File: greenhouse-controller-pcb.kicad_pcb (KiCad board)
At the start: 2 copper layers, 1 part, among them J4 JTAG Interface

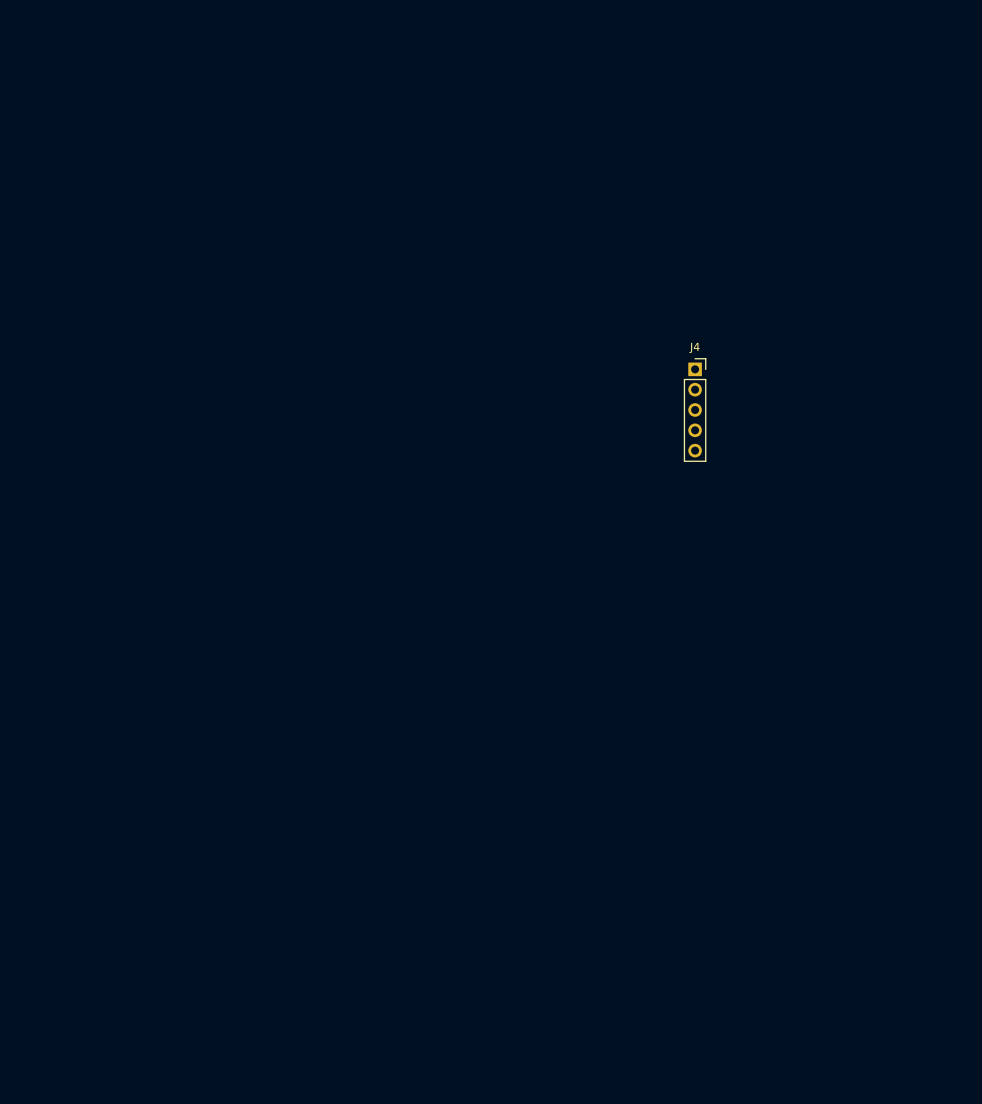
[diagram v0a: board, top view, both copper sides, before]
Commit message: version 1
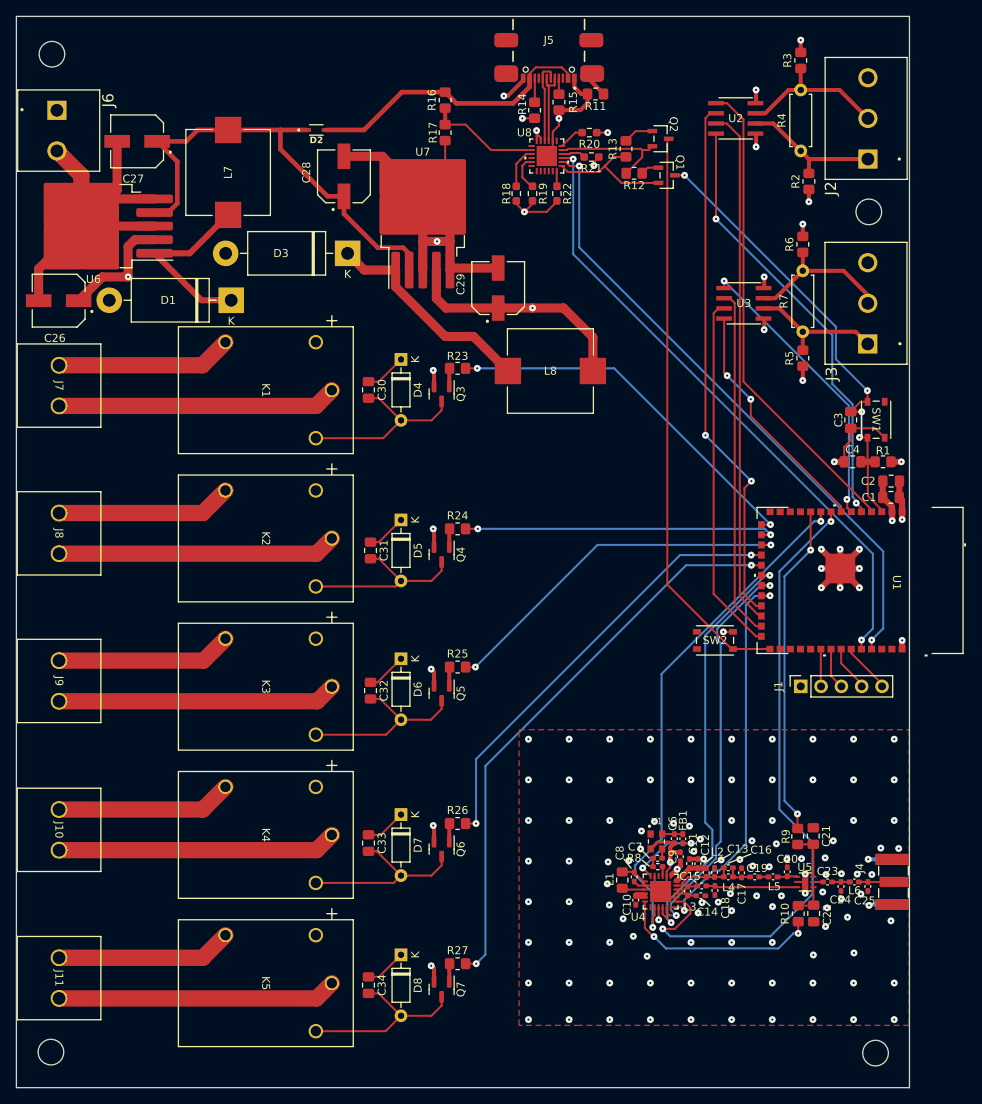
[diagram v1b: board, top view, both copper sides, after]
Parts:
- added C1: 22uF, Capacitor_SMD:C_0805_2012Metric_Pad1.18x1.45mm_HandSolder, F.Cu at (189.6, 87.1)
- added C10: 100nF, Capacitor_SMD:C_0402_1005Metric_Pad0.74x0.62mm_HandSolder, F.Cu at (157.7, 137.5)
- added C11: 47nF, Capacitor_SMD:C_0402_1005Metric_Pad0.74x0.62mm_HandSolder, F.Cu at (164.4, 132.9)
- added C12: 47pF, Capacitor_SMD:C_0402_1005Metric_Pad0.74x0.62mm_HandSolder, F.Cu at (165.4, 132.9)
- added C13: 8.2pF, Capacitor_SMD:C_0402_1005Metric_Pad0.74x0.62mm_HandSolder, F.Cu at (167.5, 134.0)
- added C14: 1.8pF, Capacitor_SMD:C_0402_1005Metric_Pad0.74x0.62mm_HandSolder, F.Cu at (165.8, 136.9)
- added C15: 2.4pF, Capacitor_SMD:C_0402_1005Metric_Pad0.74x0.62mm_HandSolder, F.Cu at (165.9, 135.7)
- added C16: 3.3pF, Capacitor_SMD:C_0402_1005Metric_Pad0.74x0.62mm_HandSolder, F.Cu at (169.3, 133.4)
- added C17: 8.2pF, Capacitor_SMD:C_0402_1005Metric_Pad0.74x0.62mm_HandSolder, F.Cu at (170.9, 134.1)
- added C18: 1.8pF, Capacitor_SMD:C_0402_1005Metric_Pad0.74x0.62mm_HandSolder, F.Cu at (167.6, 136.3)
- added C19: 39pF, Capacitor_SMD:C_0402_1005Metric_Pad0.74x0.62mm_HandSolder, F.Cu at (172.6, 134.6)
- added C2: 0.1uF, Capacitor_SMD:C_0805_2012Metric_Pad1.18x1.45mm_HandSolder, F.Cu at (189.6, 85.1)
- added C20: 3.0pF, Capacitor_SMD:C_0402_1005Metric_Pad0.74x0.62mm_HandSolder, F.Cu at (176.6, 133.9)
- added C21: 100nF, Capacitor_SMD:C_0805_2012Metric_Pad1.18x1.45mm_HandSolder, F.Cu at (179.9, 129.5)
- added C22: 100nF, Capacitor_SMD:C_0805_2012Metric_Pad1.18x1.45mm_HandSolder, F.Cu at (179.9, 139.1)
- added C23: 39pF, Capacitor_SMD:C_0402_1005Metric_Pad0.74x0.62mm_HandSolder, F.Cu at (181.7, 135.2)
- added C24: 3.3pF, Capacitor_SMD:C_0402_1005Metric_Pad0.74x0.62mm_HandSolder, F.Cu at (183.3, 135.8)
- added C25: 3.3pF, Capacitor_SMD:C_0402_1005Metric_Pad0.74x0.62mm_HandSolder, F.Cu at (186.7, 135.8)
- added C26: 120 uF, Library:CAP_EEEFNV121XUP, F.Cu at (85.5, 62.5)
- added C27: 120 uF, Library:CAP_EEEFNV121XUP, F.Cu at (95.4, 42.6)
- added C28: 120 uF, Library:CAP_EEEFNV121XUP, F.Cu at (121.2, 47.0)
- added C29: 120 uF, Library:CAP_EEEFNV121XUP, F.Cu at (140.5, 61.0)
- added C3: 1uF, Capacitor_SMD:C_0805_2012Metric_Pad1.18x1.45mm_HandSolder, F.Cu at (184.6, 77.4)
- added C30: 0.1 uF, Capacitor_SMD:C_0805_2012Metric_Pad1.18x1.45mm_HandSolder, F.Cu at (124.3, 73.7)
- added C31: 0.1 uF, Capacitor_SMD:C_0805_2012Metric_Pad1.18x1.45mm_HandSolder, F.Cu at (124.5, 93.8)
- added C32: 0.1 uF, Capacitor_SMD:C_0805_2012Metric_Pad1.18x1.45mm_HandSolder, F.Cu at (124.5, 111.3)
- added C33: 0.1 uF, Capacitor_SMD:C_0805_2012Metric_Pad1.18x1.45mm_HandSolder, F.Cu at (124.3, 130.3)
- added C34: 0.1 uF, Capacitor_SMD:C_0805_2012Metric_Pad1.18x1.45mm_HandSolder, F.Cu at (124.3, 148.1)
- added C4: 0.1uF, Capacitor_SMD:C_0805_2012Metric_Pad1.18x1.45mm_HandSolder, F.Cu at (184.8, 82.7)
- added C6: 100nF, Capacitor_SMD:C_0402_1005Metric_Pad0.74x0.62mm_HandSolder, F.Cu at (162.5, 129.8)
- added C7: 10pF, Capacitor_SMD:C_0402_1005Metric_Pad0.74x0.62mm_HandSolder, F.Cu at (160.4, 132.2)
- added C8: 470nF, Capacitor_SMD:C_0402_1005Metric_Pad0.74x0.62mm_HandSolder, F.Cu at (157.5, 134.6)
- added C9: 10nF, Capacitor_SMD:C_0402_1005Metric_Pad0.74x0.62mm_HandSolder, F.Cu at (163.3, 132.0)
- added D1: 1N5822, Diode_THT:D_DO-201AD_P15.24mm_Horizontal, F.Cu at (107.1, 62.5)
- added D2: BAT760-7, Library:SOD2513X120N, F.Cu at (117.8, 41.2)
- added D3: 1N5822, Diode_THT:D_DO-201AD_P15.24mm_Horizontal, F.Cu at (121.7, 56.6)
- added D4: 1N4148, Diode_THT:D_DO-35_SOD27_P7.62mm_Horizontal, F.Cu at (128.3, 69.9)
- added D5: 1N4148, Diode_THT:D_DO-35_SOD27_P7.62mm_Horizontal, F.Cu at (128.3, 89.9)
- added D6: 1N4148, Diode_THT:D_DO-35_SOD27_P7.62mm_Horizontal, F.Cu at (128.3, 107.3)
- added D7: 1N4148, Diode_THT:D_DO-35_SOD27_P7.62mm_Horizontal, F.Cu at (128.3, 126.8)
- added D8: 1N4148, Diode_THT:D_DO-35_SOD27_P7.62mm_Horizontal, F.Cu at (128.3, 144.3)
- added FB1: 10Ω@100MHz, Inductor_SMD:L_0402_1005Metric_Pad0.77x0.64mm_HandSolder, F.Cu at (163.6, 129.8)
- added J1: JTAG Interface, Connector_PinSocket_2.54mm:PinSocket_1x05_P2.54mm_Vertical, F.Cu at (178.3, 110.7)
- added J10: Relay 5 Ctrl., Library:TB004-508-02BE_CUD, F.Cu at (85.6, 126.1)
- added J11: Relay 3 Ctrl., Library:TB004-508-02BE_CUD, F.Cu at (85.6, 144.7)
- added J2: Screw_Terminal_01x03, Library:CUI_TB007-508-03BE, F.Cu at (186.7, 44.8)
- added J3: Screw_Terminal_01x03, Library:CUI_TB007-508-03BE, F.Cu at (186.7, 67.9)
- added J5: USB4105GFA, Library:GCT_USB4105GFA, F.Cu at (146.8, 30.0)
- added J6: POWER IN, Library:CUI_TB007-508-02BE, F.Cu at (85.3, 38.7)
- added J7: Relay 1 Ctrl., Library:TB004-508-02BE_CUD, F.Cu at (85.6, 70.6)
- added J8: Relay 4 Ctrl., Library:TB004-508-02BE_CUD, F.Cu at (85.6, 89.1)
- added J9: Relay 2 Ctrl., Library:TB004-508-02BE_CUD, F.Cu at (85.6, 107.5)
- added K1: G5LE-1A4 DC12, Library:RELAY_G5LE-1A DC5_OMR, F.Cu at (103.2, 73.7)
- added K2: G5LE-1A4 DC12, Library:RELAY_G5LE-1A DC5_OMR, F.Cu at (103.2, 92.3)
- added K3: G5LE-1A4 DC12, Library:RELAY_G5LE-1A DC5_OMR, F.Cu at (103.2, 110.8)
- added K4: G5LE-1A4 DC12, Library:RELAY_G5LE-1A DC5_OMR, F.Cu at (103.2, 129.3)
- added K5: G5LE-1A4 DC12, Library:RELAY_G5LE-1A DC5_OMR, F.Cu at (103.2, 147.8)
- added L1: 15uH, Inductor_SMD:L_0805_2012Metric_Pad1.15x1.40mm_HandSolder, F.Cu at (156.0, 135.0)
- added L2: 47nH, Inductor_SMD:L_0402_1005Metric_Pad0.77x0.64mm_HandSolder, F.Cu at (166.5, 134.0)
- added L3: 15nH, Inductor_SMD:L_0402_1005Metric_Pad0.77x0.64mm_HandSolder, F.Cu at (164.2, 136.3)
- added L4: 2.2nH, Inductor_SMD:L_0402_1005Metric_Pad0.77x0.64mm_HandSolder, F.Cu at (169.3, 134.6)
- added L5: 9.1nH, Inductor_SMD:L_0402_1005Metric_Pad0.77x0.64mm_HandSolder, F.Cu at (174.8, 134.6)
- added L6: 9.1nH, Inductor_SMD:L_0402_1005Metric_Pad0.77x0.64mm_HandSolder, F.Cu at (185.0, 135.2)
- added L7: 68 uH, Library:DR1050, F.Cu at (106.7, 46.5)
- added L8: 68 uH, Library:DR1050, F.Cu at (147.0, 71.3)
- added Q1: SS8050-G, Library:TRAN_SS8050-G_CIP, F.Cu at (161.5, 46.9)
- added Q2: SS8050-G, Library:TRAN_SS8050-G_CIP, F.Cu at (160.8, 42.3)
- added Q3: 2N7002, Package_TO_SOT_SMD:SOT-23, F.Cu at (133.4, 74.2)
- added Q4: 2N7002, Package_TO_SOT_SMD:SOT-23, F.Cu at (133.4, 94.3)
- added Q5: 2N7002, Package_TO_SOT_SMD:SOT-23, F.Cu at (133.4, 111.6)
- added Q6: 2N7002, Package_TO_SOT_SMD:SOT-23, F.Cu at (133.4, 131.1)
- added Q7: 2N7002, Package_TO_SOT_SMD:SOT-23, F.Cu at (133.4, 148.6)
- added R1: 10kΩ, Resistor_SMD:R_0805_2012Metric_Pad1.20x1.40mm_HandSolder, F.Cu at (188.6, 82.7)
- added R10: 100Ω, Resistor_SMD:R_0805_2012Metric_Pad1.20x1.40mm_HandSolder, F.Cu at (178.0, 139.2)
- added R11: 1MΩ, Resistor_SMD:R_0805_2012Metric_Pad1.20x1.40mm_HandSolder, F.Cu at (152.7, 36.7)
- added R12: 10k, Resistor_SMD:R_0805_2012Metric_Pad1.20x1.40mm_HandSolder, F.Cu at (157.5, 46.6)
- added R13: 10k, Resistor_SMD:R_0805_2012Metric_Pad1.20x1.40mm_HandSolder, F.Cu at (156.5, 43.6)
- added R14: 5.11kΩ, Resistor_SMD:R_0805_2012Metric_Pad1.20x1.40mm_HandSolder, F.Cu at (145.0, 38.7)
- added R15: 5.11kΩ, Resistor_SMD:R_0805_2012Metric_Pad1.20x1.40mm_HandSolder, F.Cu at (148.1, 37.7)
- added R16: 22.1kΩ, Resistor_SMD:R_0805_2012Metric_Pad1.20x1.40mm_HandSolder, F.Cu at (133.9, 37.5)
- added R17: 47.5kΩ, Resistor_SMD:R_0805_2012Metric_Pad1.20x1.40mm_HandSolder, F.Cu at (133.9, 41.5)
- added R18: 2kΩ, Resistor_SMD:R_0603_1608Metric_Pad0.98x0.95mm_HandSolder, F.Cu at (142.7, 49.1)
- added R19: 2kΩ, Resistor_SMD:R_0603_1608Metric_Pad0.98x0.95mm_HandSolder, F.Cu at (144.8, 49.1)
- added R2: 1k, Resistor_SMD:R_0805_2012Metric_Pad1.20x1.40mm_HandSolder, F.Cu at (179.3, 47.6)
- added R20: 2kΩ, Resistor_SMD:R_0603_1608Metric_Pad0.98x0.95mm_HandSolder, F.Cu at (151.9, 41.5)
- added R21: 2kΩ, Resistor_SMD:R_0603_1608Metric_Pad0.98x0.95mm_HandSolder, F.Cu at (152.1, 44.6)
- added R22: 2kΩ, Resistor_SMD:R_0603_1608Metric_Pad0.98x0.95mm_HandSolder, F.Cu at (147.8, 49.1)
- added R23: 100Ω, Resistor_SMD:R_0805_2012Metric_Pad1.20x1.40mm_HandSolder, F.Cu at (135.4, 71.0)
- added R24: 100Ω, Resistor_SMD:R_0805_2012Metric_Pad1.20x1.40mm_HandSolder, F.Cu at (135.4, 91.1)
- added R25: 100Ω, Resistor_SMD:R_0805_2012Metric_Pad1.20x1.40mm_HandSolder, F.Cu at (135.4, 108.3)
- added R26: 100Ω, Resistor_SMD:R_0805_2012Metric_Pad1.20x1.40mm_HandSolder, F.Cu at (135.4, 127.9)
- added R27: 100Ω, Resistor_SMD:R_0805_2012Metric_Pad1.20x1.40mm_HandSolder, F.Cu at (135.4, 145.4)
- added R3: 1k, Resistor_SMD:R_0805_2012Metric_Pad1.20x1.40mm_HandSolder, F.Cu at (178.3, 32.5)
- added R4: 120, Resistor_THT:R_Axial_DIN0207_L6.3mm_D2.5mm_P7.62mm_Horizontal, F.Cu at (178.3, 43.8)
- added R5: 1k, Resistor_SMD:R_0805_2012Metric_Pad1.20x1.40mm_HandSolder, F.Cu at (178.6, 69.7)
- added R6: 1k, Resistor_SMD:R_0805_2012Metric_Pad1.20x1.40mm_HandSolder, F.Cu at (178.6, 55.5)
- added R7: 120, Resistor_THT:R_Axial_DIN0207_L6.3mm_D2.5mm_P7.62mm_Horizontal, F.Cu at (178.6, 66.4)
- added R8: 220Ω, Resistor_SMD:R_0402_1005Metric_Pad0.72x0.64mm_HandSolder, F.Cu at (160.4, 133.3)
- added R9: 100Ω, Resistor_SMD:R_0805_2012Metric_Pad1.20x1.40mm_HandSolder, F.Cu at (177.9, 129.5)
- added REF**: MountingHole_3.2mm_M3, MountingHole:MountingHole_3.2mm_M3, F.Cu at (187.7, 156.6)
- added REF**: MountingHole_3.2mm_M3, MountingHole:MountingHole_3.2mm_M3, F.Cu at (186.8, 51.4)
- added REF**: MountingHole_3.2mm_M3, MountingHole:MountingHole_3.2mm_M3, F.Cu at (84.6, 156.5)
- added REF**: MountingHole_3.2mm_M3, MountingHole:MountingHole_3.2mm_M3, F.Cu at (84.7, 31.7)
- added SW1: RESET, Library:SW4_PTS815 SJM 250 SMTR LFS_CNK, F.Cu at (187.7, 77.4)
- added SW2: Boot mode, Library:SW4_PTS815 SJM 250 SMTR LFS_CNK, F.Cu at (167.6, 105.0)
- added U1: ~, Library:ESP32-S3-WROOM-1_EXP, F.Cu at (185.7, 97.5)
- added U2: ADM3483ARZ, Library:R_8_ADI, F.Cu at (170.2, 39.8)
- added U3: ADM3483ARZ, Library:R_8_ADI, F.Cu at (171.2, 62.9)
- added U4: SX1262IMLTRT, Library:QFN24_4X4_SEM, F.Cu at (160.8, 136.4)
- added U5: CG2179M2, Library:MINISO6_CG21_CEL, F.Cu at (178.9, 135.2)
- added U6: LM2595S-5, Package_TO_SOT_SMD:TO-263-5_TabPin3, F.Cu at (89.9, 53.2)
- added U7: LM2595S-3.3, Package_TO_SOT_SMD:TO-263-5_TabPin3, F.Cu at (131.1, 51.1)
- added U8: CP2102N-A02-GQFN24R, Library:QFN24_SIL, F.Cu at (146.6, 44.5)
- added Y1: 32 MHz, Library:OSC_ECS-TXO-2520-33-320-AN-TR, F.Cu at (160.3, 130.1)
- J4: value JTAG Interface -> SMA; footprint Connector_PinSocket_2.54mm:PinSocket_1x05_P2.54mm_Vertical -> Connector_Coaxial:SMA_Samtec_SMA-J-P-X-ST-EM1_EdgeMount
- moved J4 68.6 mm to (189.8, 135.2), turned to 90 degrees
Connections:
- J4 pad 1: GNDREF -> Net-(J4-In)
- J4 pad 2: /JTAG_TCK -> GNDREF
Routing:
- net GNDREF: track 0.00 -> 211.1 mm, vias 0 -> 135
- net LoRa_SPI_CS: track 0.00 -> 80.6 mm, vias 0 -> 2
- net ESP32_UART_TX: track 0.00 -> 79.1 mm, vias 0 -> 2
- net ESP32_UART_RX: track 0.00 -> 78.8 mm, vias 0 -> 2
- net BOOT_MODE: track 0.00 -> 72.0 mm
- net RELAY_5: track 0.00 -> 71.4 mm, vias 0 -> 2
- net RS-485_1_RX_EN: track 0.00 -> 66.5 mm, vias 0 -> 2
- net LoRa_BUSY: track 0.00 -> 65.6 mm, vias 0 -> 2
- net RS-485_1_TX_EN: track 0.00 -> 64.9 mm
- net RS-485_1_RX: track 0.00 -> 59.9 mm
- net +3.3V: track 0.00 -> 59.3 mm, vias 0 -> 13
- net EN: track 0.00 -> 59.1 mm, vias 0 -> 4
- net +5V: track 0.00 -> 58.7 mm
- net RELAY_4: track 0.00 -> 55.6 mm, vias 0 -> 2
- net RS-485_1_TX: track 0.00 -> 54.8 mm, vias 0 -> 2
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- added copper zone on In2.Cu, net +12V
- added copper zone on In2.Cu, net +3.3V
- added copper zone on F.Cu, net GNDREF
- added copper zone on In1.Cu, net GNDREF
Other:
- board outline added: 111.6 x 133.9 mm
- copper layers 2 -> 4
